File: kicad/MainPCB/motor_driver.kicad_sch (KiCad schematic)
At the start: 36 parts

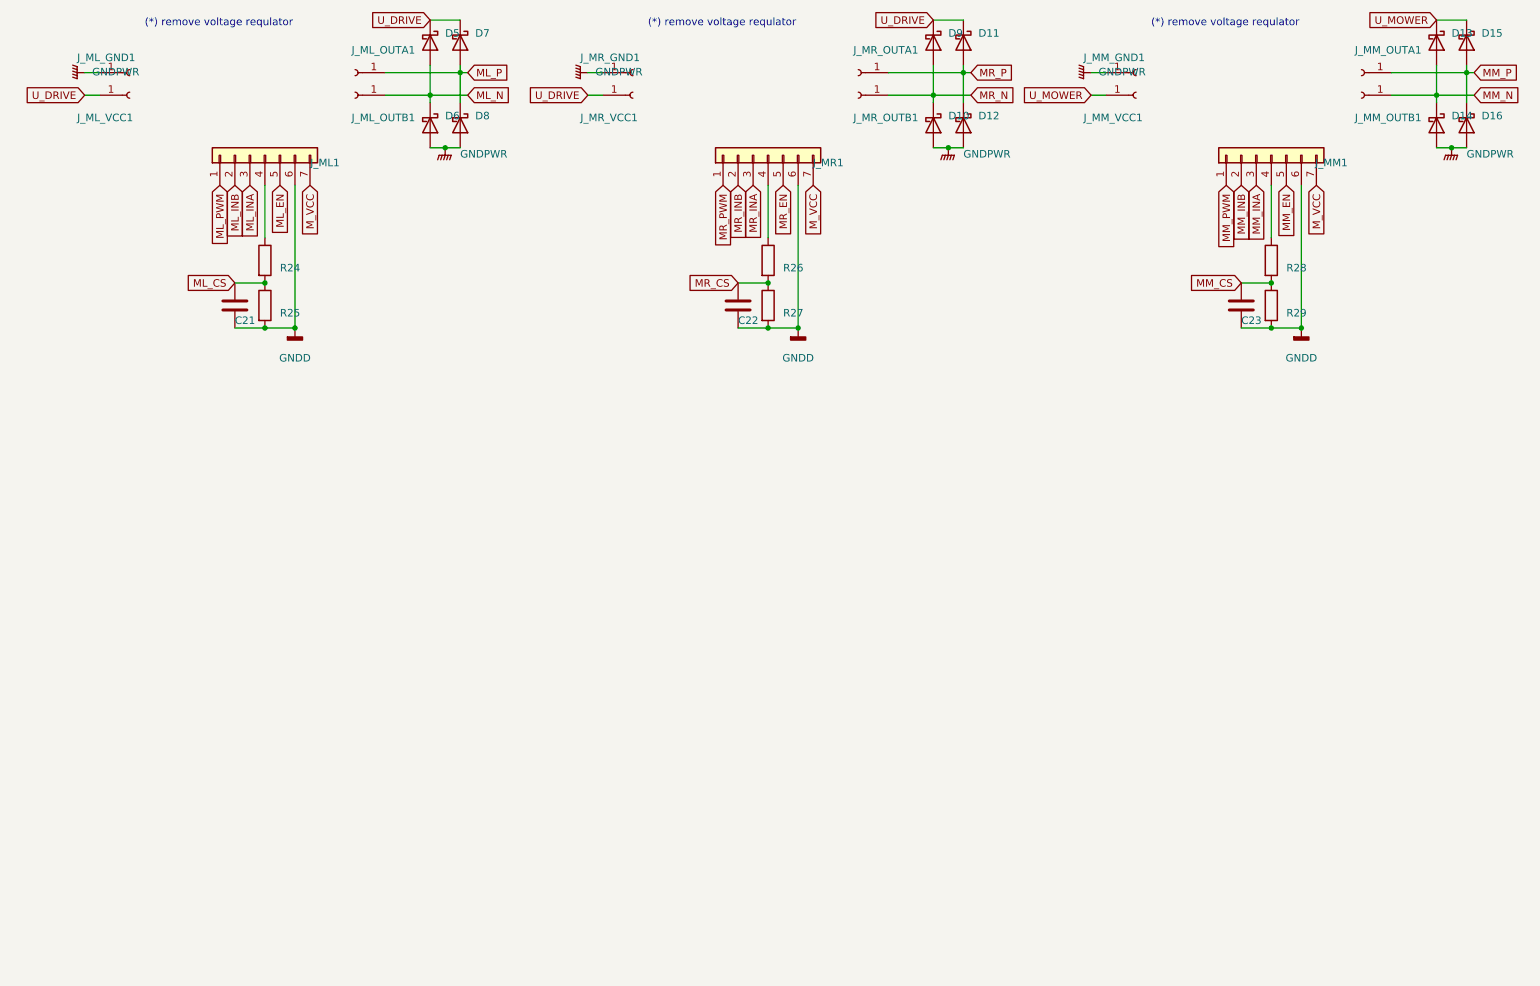
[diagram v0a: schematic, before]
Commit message: some further progress
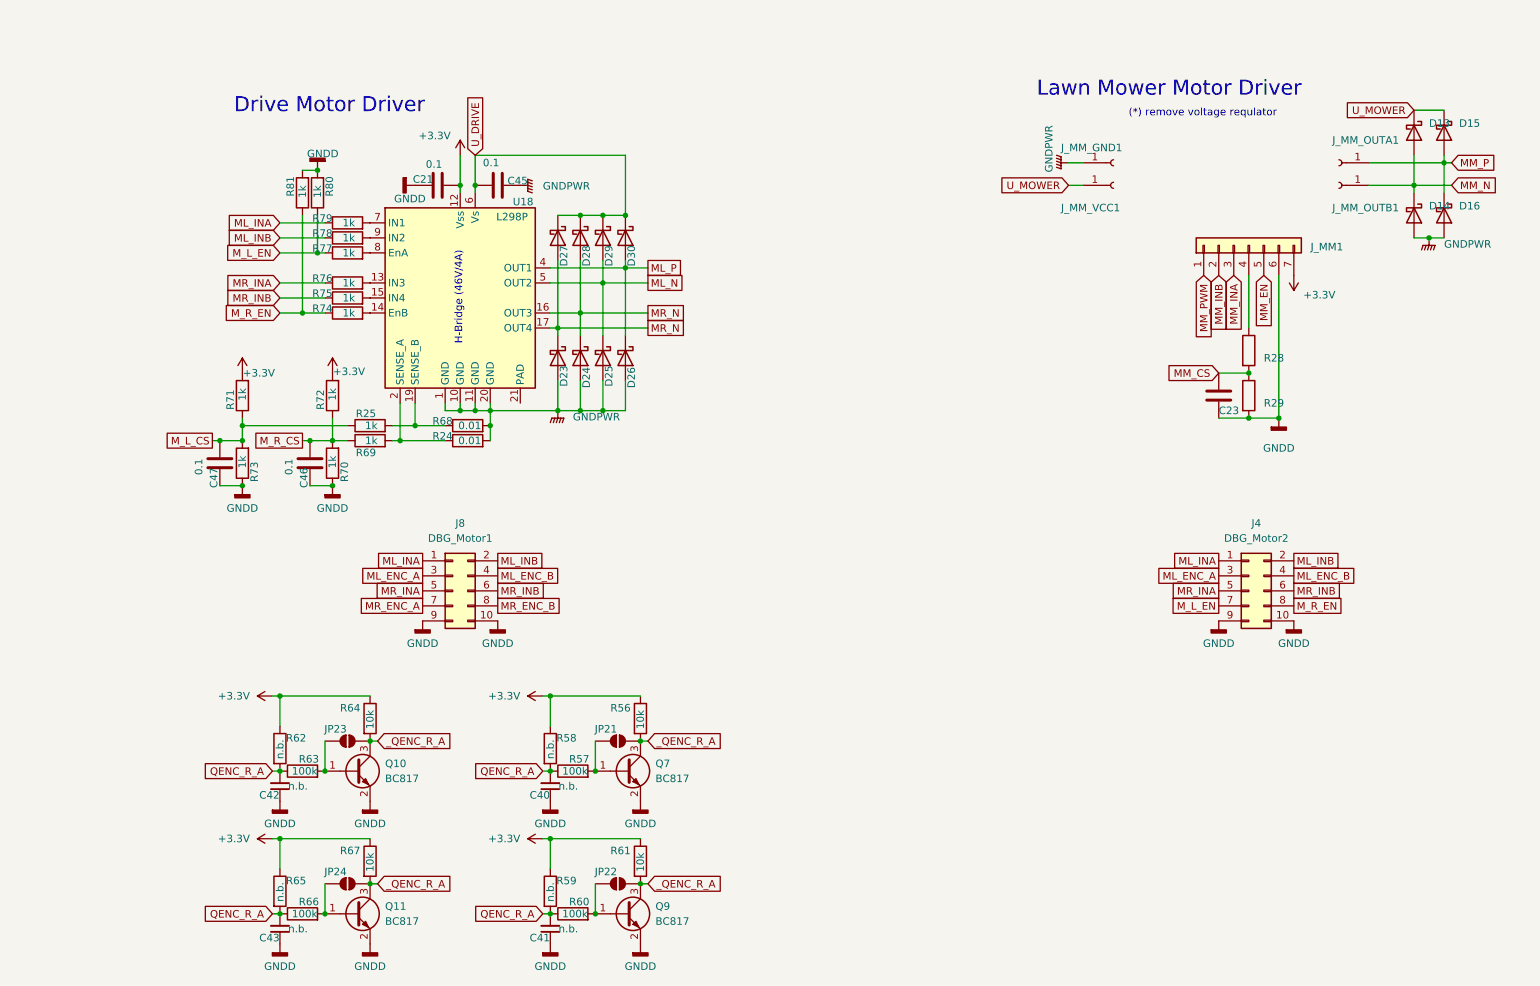
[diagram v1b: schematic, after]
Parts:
- removed C22: ~, Capacitor_SMD:C_0805_2012Metric_Pad1.18x1.45mm_HandSolder, symbol Device:C
- removed D10, D11, D12, D5, D6, D7, D8, D9: ~, Diode_SMD:D_SMA_Handsoldering, symbol Diode:MBRA340
- removed J_ML1: Conn_01x07, Connector_PinSocket_2.54mm:PinSocket_1x07_P2.54mm_Vertical, symbol Connector_Generic:Conn_01x07
- removed J_ML_GND1, J_ML_OUTA1, J_ML_OUTB1, J_ML_VCC1, J_MR_GND1, J_MR_OUTA1, J_MR_OUTB1, J_MR_VCC1: ~, Connector_Wire:SolderWire-1sqmm_1x01_D1.4mm_OD2.7mm, symbol Connector:Conn_01x01_Female
- removed J_MR1: ~, Connector_PinSocket_2.54mm:PinSocket_1x07_P2.54mm_Vertical, symbol Connector_Generic:Conn_01x07
- removed R26, R27: ~, Resistor_SMD:R_0805_2012Metric_Pad1.20x1.40mm_HandSolder, symbol Device:R
- added C40, C41, C42, C43: n.b., symbol Device:C_Small
- added C45, C46, C47: 0.1, Capacitor_SMD:C_0805_2012Metric_Pad1.18x1.45mm_HandSolder, symbol Device:C
- added D23, D24, D25, D26, D27, D28, D29, D30: ~, Diode_SMD:D_SMA_Handsoldering, symbol Diode:MBRA340
- added J4: DBG_Motor2, symbol Connector_Generic:Conn_02x05_Odd_Even
- added J8: DBG_Motor1, symbol Connector_Generic:Conn_02x05_Odd_Even
- added JP21, JP22, JP23, JP24: SolderJumper_2_Open, symbol Jumper:SolderJumper_2_Open
- added Q10, Q11, Q7, Q9: BC817, Package_TO_SOT_SMD:SOT-23, symbol Transistor_BJT:BC817
- added R56, R61, R64, R67: 10k, Resistor_SMD:R_0805_2012Metric, symbol Device:R
- added R57, R60, R63, R66: 100k, Resistor_SMD:R_0805_2012Metric, symbol Device:R
- added R58, R59, R62, R65: n.b., Resistor_SMD:R_0805_2012Metric, symbol Device:R
- added R68: 0.01, Resistor_SMD:R_0805_2012Metric_Pad1.20x1.40mm_HandSolder, symbol Device:R
- added R69, R70, R71, R72, R73, R74, R75, R76, R77, R78, R79, R80, R81: 1k, Resistor_SMD:R_0805_2012Metric_Pad1.20x1.40mm_HandSolder, symbol Device:R
- added U18: L298P, Package_SO:HSOP-20-1EP_11.0x15.9mm_P1.27mm_SlugDown, symbol Driver_Motor:L298P
- C21: value ~ -> 0.1
- R24: value ~ -> 0.01
- R25: value ~ -> 1k
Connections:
- net GNDD: now also C21.1, C40.1, C41.1, C42.1, C43.1, C46.1, C47.1, J4.10 (Pin_10), J4.9 (Pin_9), J8.10 (Pin_10), J8.9 (Pin_9), Q10.2 (E), Q11.2 (E), Q7.2 (E), Q9.2 (E), R70.1, R73.1, R80.2, R81.2; no longer C21.2, R25.2
- net GNDPWR: now also R24.2, C45.2, D23.2 (A), D24.2 (A), D25.2 (A), D26.2 (A), R68.2, U18.1 (GND), U18.10 (GND), U18.11 (GND), U18.20 (GND)
- net ML_INA: now also J4.1 (Pin_1), J8.1 (Pin_1), R79.1
- net ML_INB: now also J4.2 (Pin_2), J8.2 (Pin_2), R78.1
- net ML_N: now also D25.1 (K), D29.2 (A), U18.5 (OUT2)
- net ML_P: now also D26.1 (K), D30.2 (A), U18.4 (OUT1)
- net MR_INA: now also J4.5 (Pin_5), J8.5 (Pin_5), R76.1
- net MR_INB: now also J4.6 (Pin_6), J8.6 (Pin_6), R75.1
- net MR_N: now also D23.1 (K), D24.1 (K), D27.2 (A), D28.2 (A), U18.16 (OUT3), U18.17 (OUT4)
- net U_DRIVE: now also C45.1, D27.1 (K), D28.1 (K), D29.1 (K), D30.1 (K), U18.6 (Vs)
- net at R24.1: now also R69.2, U18.2 (SENSE_A)
- removed net ML_CS: C21.1, R24.2, R25.1
- net M_VCC renamed +3.3V
- net +3.3V: now also C21.2, R56.1, R58.1, R59.1, R61.1, R62.1, R64.1, R65.1, R67.1, R71.2, R72.2, U18.12 (Vss)
- new net: R25.2, R68.1, U18.19 (SENSE_B)
- new net: R76.2, U18.13 (IN3)
- new net: R74.2, U18.14 (EnB)
- new net: R75.2, U18.15 (IN4)
- new net: R79.2, U18.7 (IN1)
- new net: R77.2, U18.8 (EnA)
- new net: R78.2, U18.9 (IN2)
- new net: JP23.1 (A), Q10.1 (B), R63.2
- new net: JP21.1 (A), Q7.1 (B), R57.2
- new net: JP24.1 (A), Q11.1 (B), R66.2
- new net: JP22.1 (A), Q9.1 (B), R60.2
- new net ML_ENC_A: J4.3 (Pin_3), J8.3 (Pin_3)
- new net ML_ENC_B: J4.4 (Pin_4), J8.4 (Pin_4)
- new net MR_ENC_A: J8.7 (Pin_7)
- new net MR_ENC_B: J8.8 (Pin_8)
- new net M_L_CS: C47.2, R25.1, R71.1, R73.2
- new net M_L_EN: J4.7 (Pin_7), R77.1, R80.1
- new net M_R_CS: C46.2, R69.1, R70.2, R72.1
- new net M_R_EN: J4.8 (Pin_8), R74.1, R81.1
- new net QENC_R_A: C40.2, C41.2, C42.2, C43.2, R57.1, R58.2, R59.2, R60.1, R62.2, R63.1, R65.2, R66.1
- new net _QENC_R_A: JP21.2 (B), JP22.2 (B), JP23.2 (B), JP24.2 (B), Q10.3 (C), Q11.3 (C), Q7.3 (C), Q9.3 (C), R56.2, R61.2, R64.2, R67.2
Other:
- note added: "Drive Motor Driver"
- note added: "H-Bridge (46V/4A)"
- note added: "Lawn Mower Motor Driver"
- moved on the sheet: C23, D13, D14, D15, D16, J_MM1, J_MM_GND1, J_MM_OUTA1, J_MM_OUTB1, J_MM_VCC1, R28, R29
